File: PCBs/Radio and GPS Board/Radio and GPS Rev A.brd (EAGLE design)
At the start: 95.9 x 90.2 mm, 7 parts

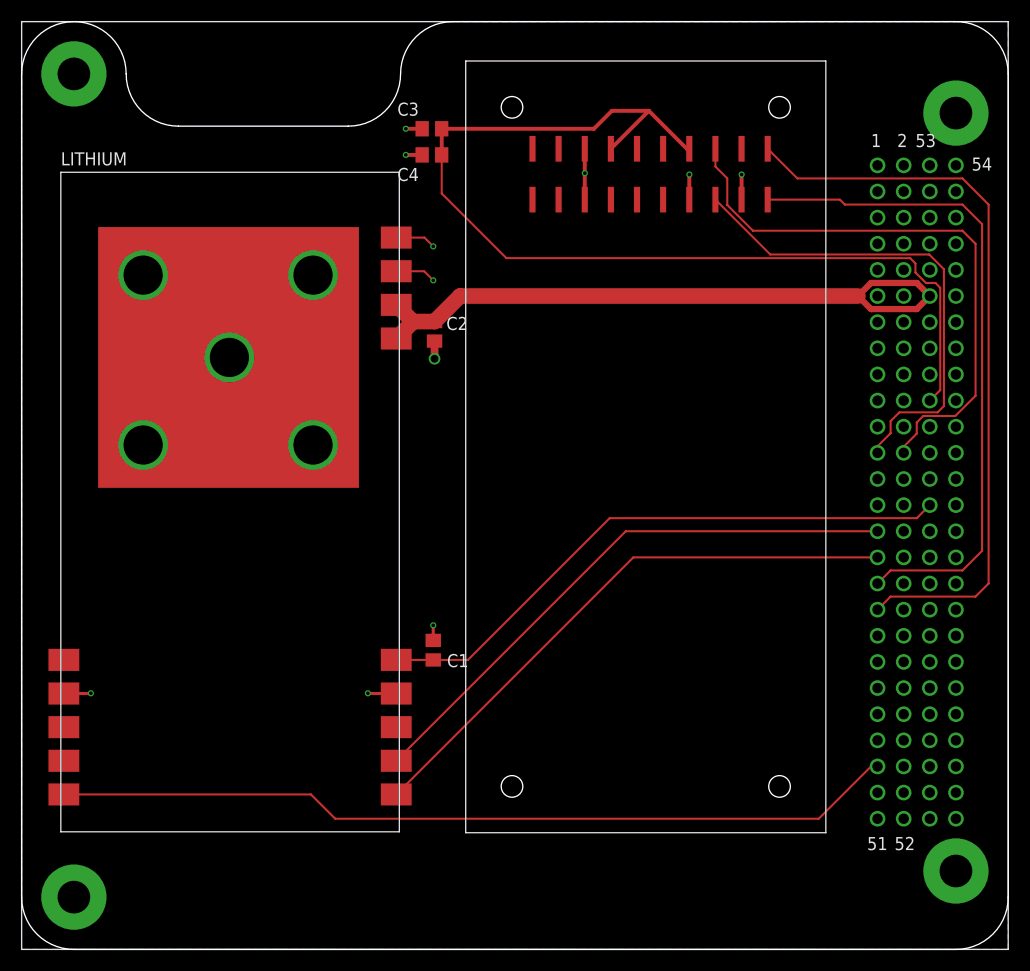
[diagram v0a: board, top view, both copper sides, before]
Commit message: So. many. changes.
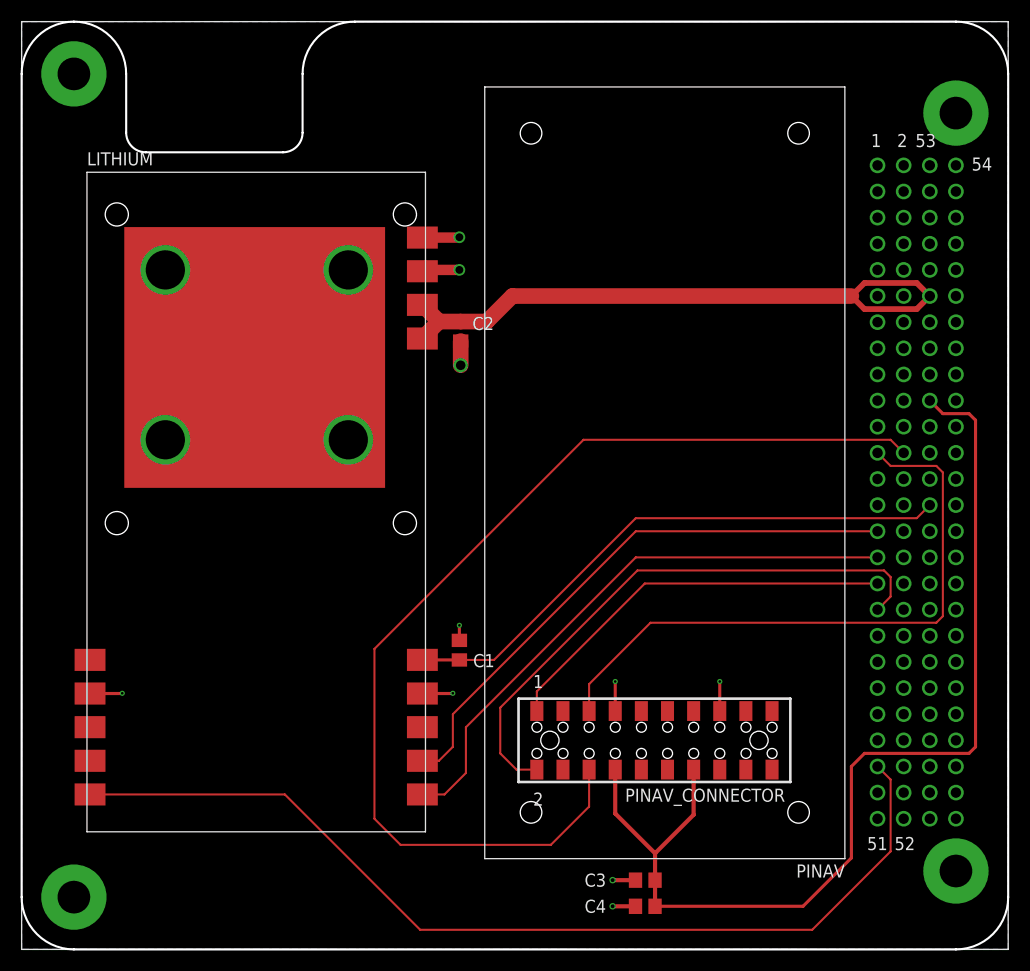
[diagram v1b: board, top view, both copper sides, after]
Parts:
- removed U$3: PC104_BOARD, PC104 Board:PC104_WITH_CSK_HEADER
- added PINAV_CONNECTOR: HLE-110-02-X-DV-BE-A, HLE-110-02-X-DV-BE-A:HLE-110-02-X-DV-BE-A
- added U$1: PC104_NO_DIMENSION, Cubesat:PC104_NO_DIMENSION
- LITHIUM: value CUBESAT_LITHIUM -> LI-1; device Radio Board Rev B:CUBESAT_LI-1 -> Cubesat:LI-1
- PINAV: value PINAVL1 -> (none); device pinavl1:PINAV-L1 -> Cubesat:PINAV-L1
- moved C3 75.9 mm to (60.6, 6.73)
- moved C4 75.9 mm to (60.6, 4.19)
- moved PINAV 40.3 mm to (80.0, 83.8), turned to 180 degrees
- moved LITHIUM 2.54 mm to (6.35, 11.4)
- moved C1 2.54 mm to (42.5, 29.1)
- moved C2 2.54 mm to (42.7, 60.1)
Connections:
- net 3V3: now also U$1.79; no longer U$3.79
- net GND: now also LITHIUM.THERM1, LITHIUM.THERM2, LITHIUM.THERM3, LITHIUM.THERM4, PINAV_CONNECTOR.15, PINAV_CONNECTOR.7, U$1.100, U$1.61, U$1.66, U$1.69, U$1.73, U$1.74, U$1.81, U$1.82, U$1.84, U$1.99; no longer PINAV.15, PINAV.16, PINAV.3, PINAV.7, U$3.100, U$3.61, U$3.66, U$3.69, U$3.73, U$3.74, U$3.81, U$3.82, U$3.84, U$3.99
- net GPS_PF: now also PINAV_CONNECTOR.6, U$1.24; no longer PINAV.6, U$3.24
- net GPS_RX: now also PINAV_CONNECTOR.2, U$1.35; no longer PINAV.2, U$3.35
- net GPS_TX: now also PINAV_CONNECTOR.1, U$1.33; no longer PINAV.1, U$3.33
- net GPS_VPP: now also PINAV_CONNECTOR.5, U$1.23; no longer PINAV.5, U$3.23
- net LI_RX: now also U$1.29; no longer U$3.29
- net LI_TX: now also U$1.31; no longer U$3.31
- net OA_RESET: now also U$1.47; no longer U$3.47
- net SW3: now also U$1.63; no longer U$3.63
- net SW9: now also PINAV_CONNECTOR.14, PINAV_CONNECTOR.8, U$1.71; no longer PINAV.14, PINAV.8, U$3.71
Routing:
- net GPS_PF: track 56.7 -> 103.9 mm
- net GPS_TX: track 65.0 -> 39.4 mm
- net GPS_RX: track 72.4 -> 56.1 mm
- net GPS_VPP: track 47.7 -> 60.8 mm
- net OA_RESET: track 82.2 -> 95.2 mm
- net SW3: track 67.0 -> 63.1 mm
- net 3V3: track 58.1 -> 55.6 mm
- net SW9: track 102.0 -> 104.3 mm
- net GND: track 29.5 -> 27.4 mm, vias 16 -> 10
- net LI_RX: track 56.0 -> 55.3 mm
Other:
- outline, holes or cut-outs redrawn
